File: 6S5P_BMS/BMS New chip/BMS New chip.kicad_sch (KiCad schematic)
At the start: 39 parts, among them J1 Screw_Terminal_01x02, J2 Screw_Terminal_01x06, Q2 AO3414, Q3 AO3414, Q4 AO3414, Q5 AO3414, Q6 AO3414, U1 MP2793DFP-0002-T, U2 MPF42792DRT-0B-0000-P, U3 LDO40LPU33RY

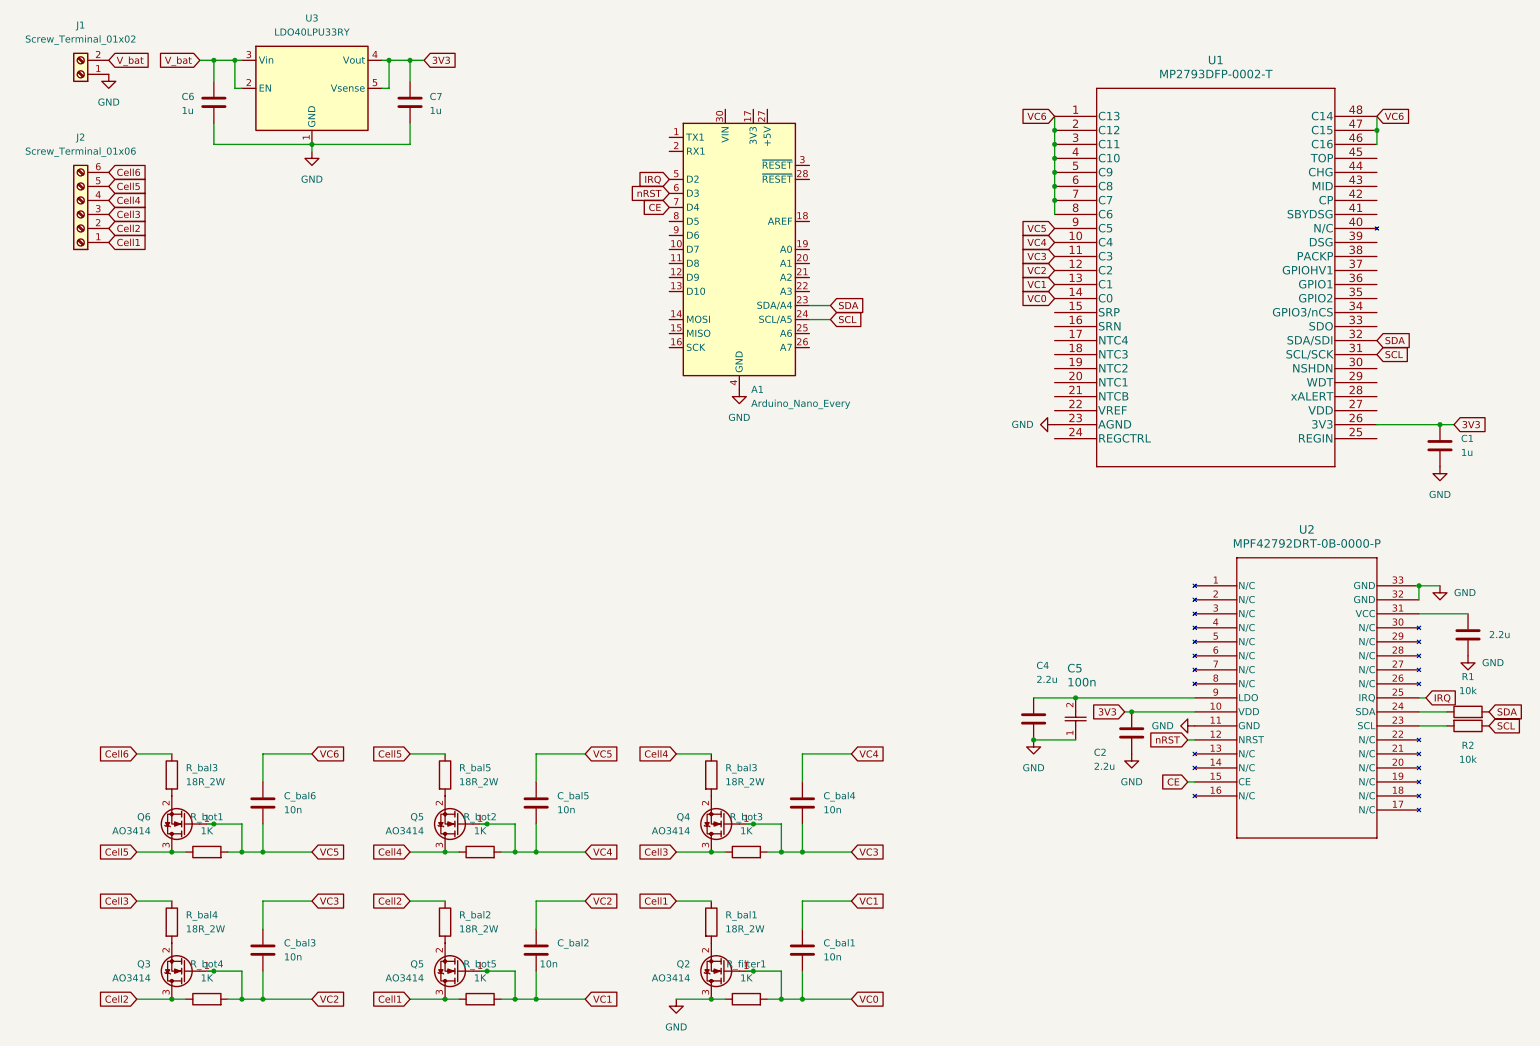
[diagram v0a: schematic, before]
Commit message: trying to restore most recent version
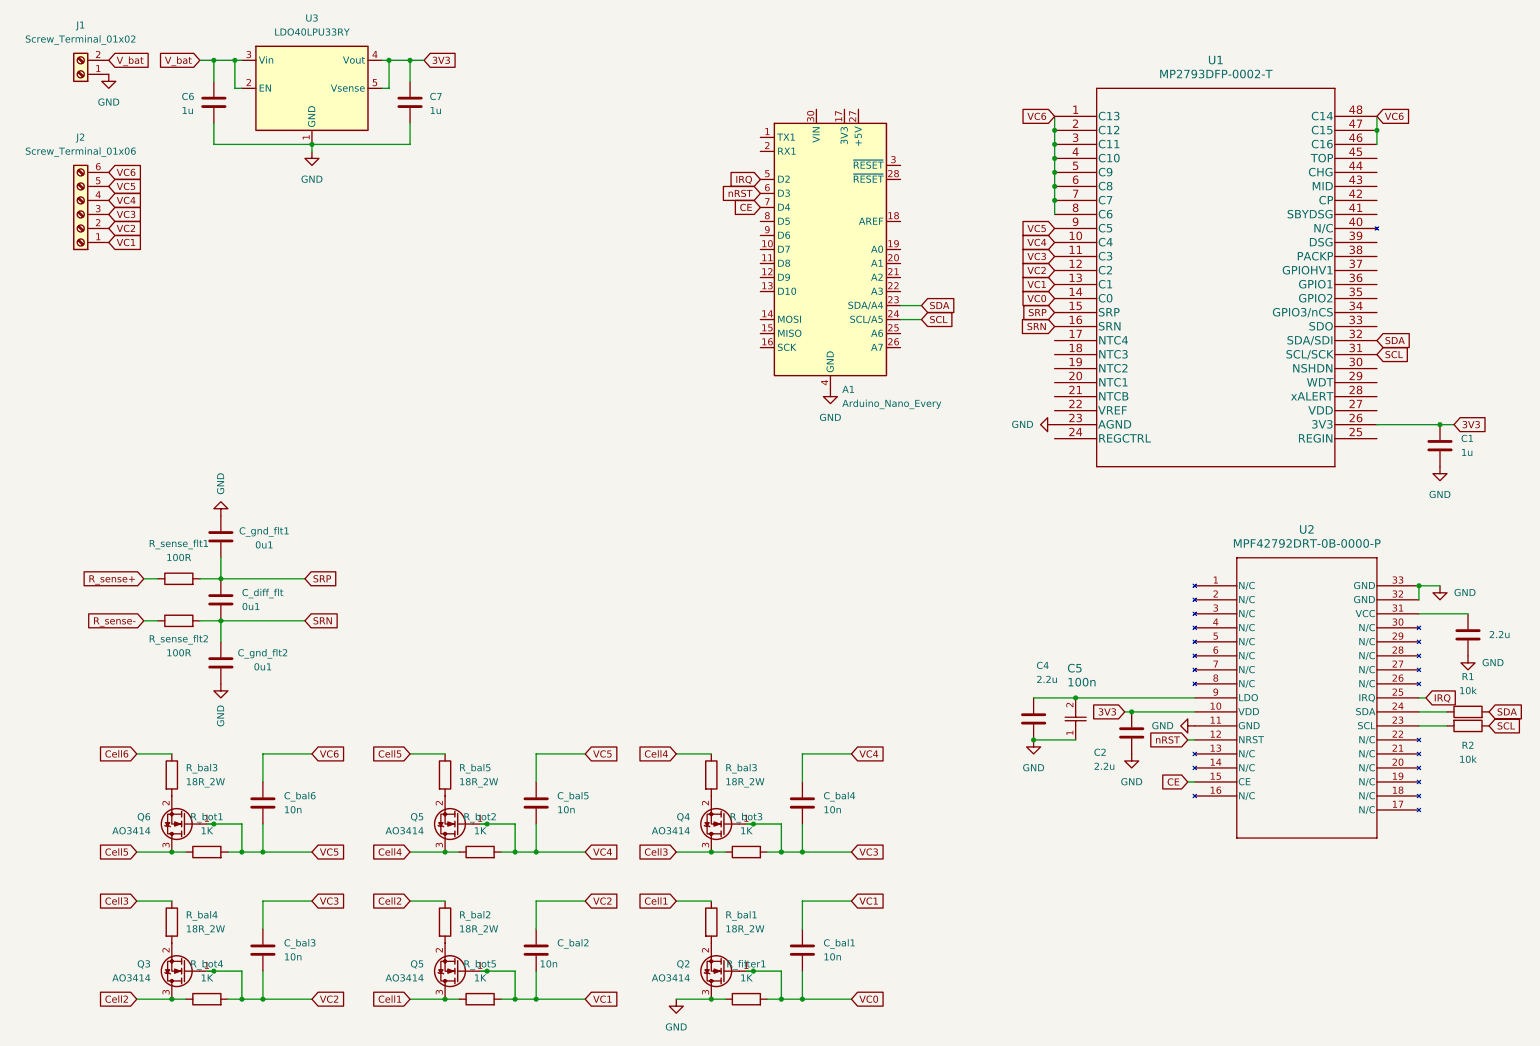
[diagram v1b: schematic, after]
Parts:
- added C_diff_flt, C_gnd_flt1, C_gnd_flt2: 0u1, rsx_capacitors:C_0603_1608Metric, symbol rsx_Capacitors:0u1
- added R_sense_flt1, R_sense_flt2: 100R, rsx_resistors:R_0603_1608Metric, symbol rsx_Resistors:100R
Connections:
- net Cell1: no longer J2.1 (Pin_1)
- net Cell2: no longer J2.2 (Pin_2)
- net Cell3: no longer J2.3 (Pin_3)
- net Cell4: no longer J2.4 (Pin_4)
- net Cell5: no longer J2.5 (Pin_5)
- net Cell6: no longer J2.6 (Pin_6)
- net GND: now also C_gnd_flt1.2, C_gnd_flt2.2
- net VC1: now also J2.1 (Pin_1)
- net VC2: now also J2.2 (Pin_2)
- net VC3: now also J2.3 (Pin_3)
- net VC4: now also J2.4 (Pin_4)
- net VC5: now also J2.5 (Pin_5)
- net VC6: now also J2.6 (Pin_6)
- net SRP: now reaches U1.15 (SRP)
- net SRP: now also C_diff_flt.1, C_gnd_flt1.1, R_sense_flt1.2
- net SRN: now reaches U1.16 (SRN)
- net SRN: now also C_diff_flt.2, C_gnd_flt2.1, R_sense_flt2.2
- new net R_sense+: R_sense_flt1.1
- new net R_sense-: R_sense_flt2.1
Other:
- moved on the sheet: A1
